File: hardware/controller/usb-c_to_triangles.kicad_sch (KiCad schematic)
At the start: 14 parts, among them J1 USB_C_Receptacle_USB2.0_16P, J2 USB_C_Receptacle_USB2.0_16P, U5 SN74LVC1T45DBV, U6 SN74LVC1T45DBV

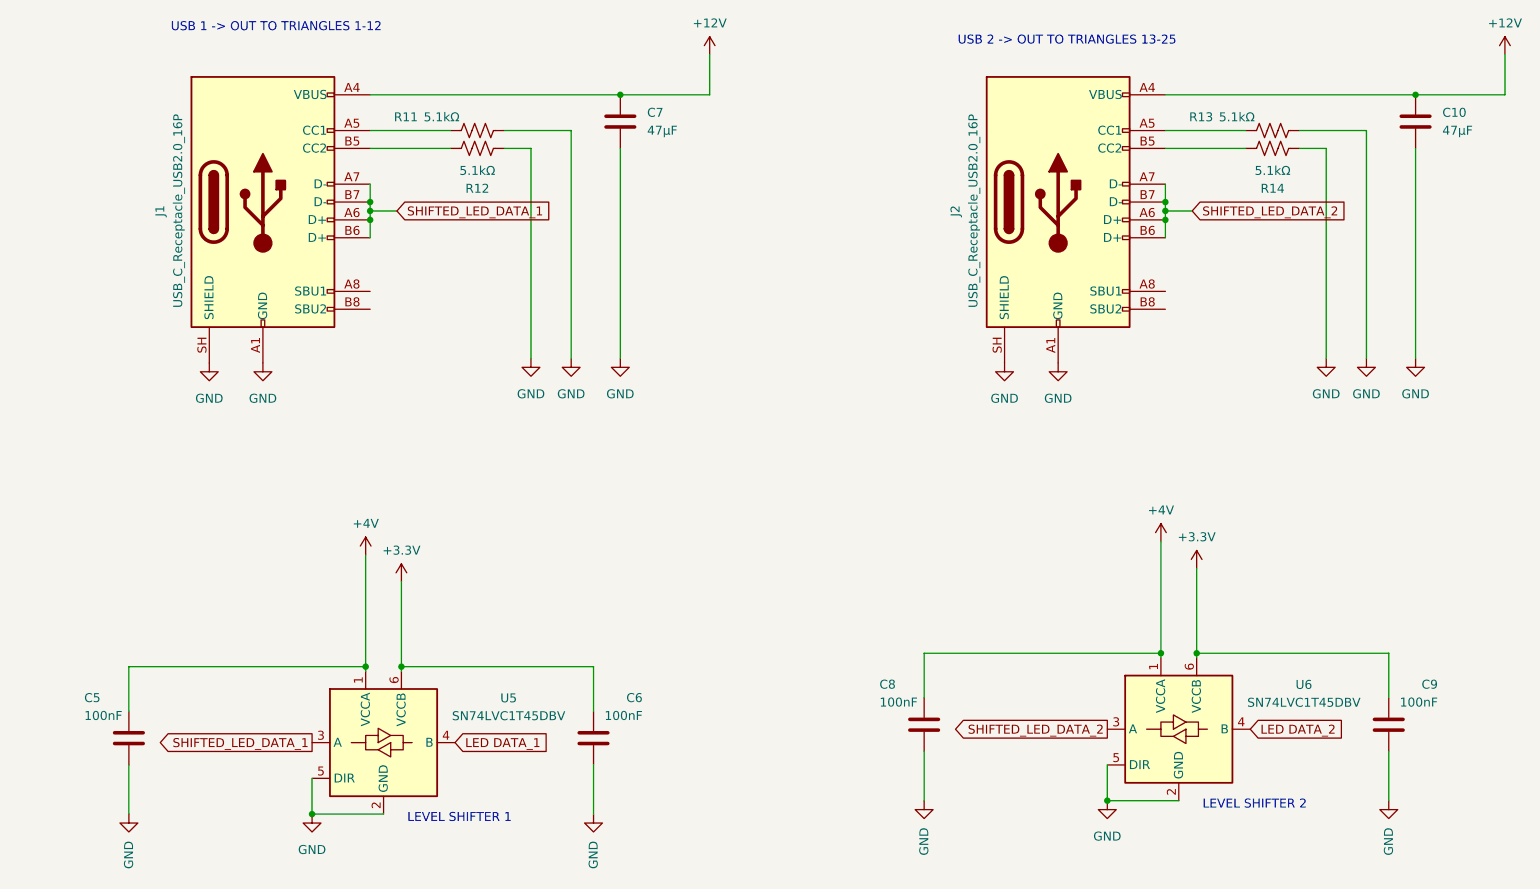
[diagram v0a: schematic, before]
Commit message: updating symbols and board
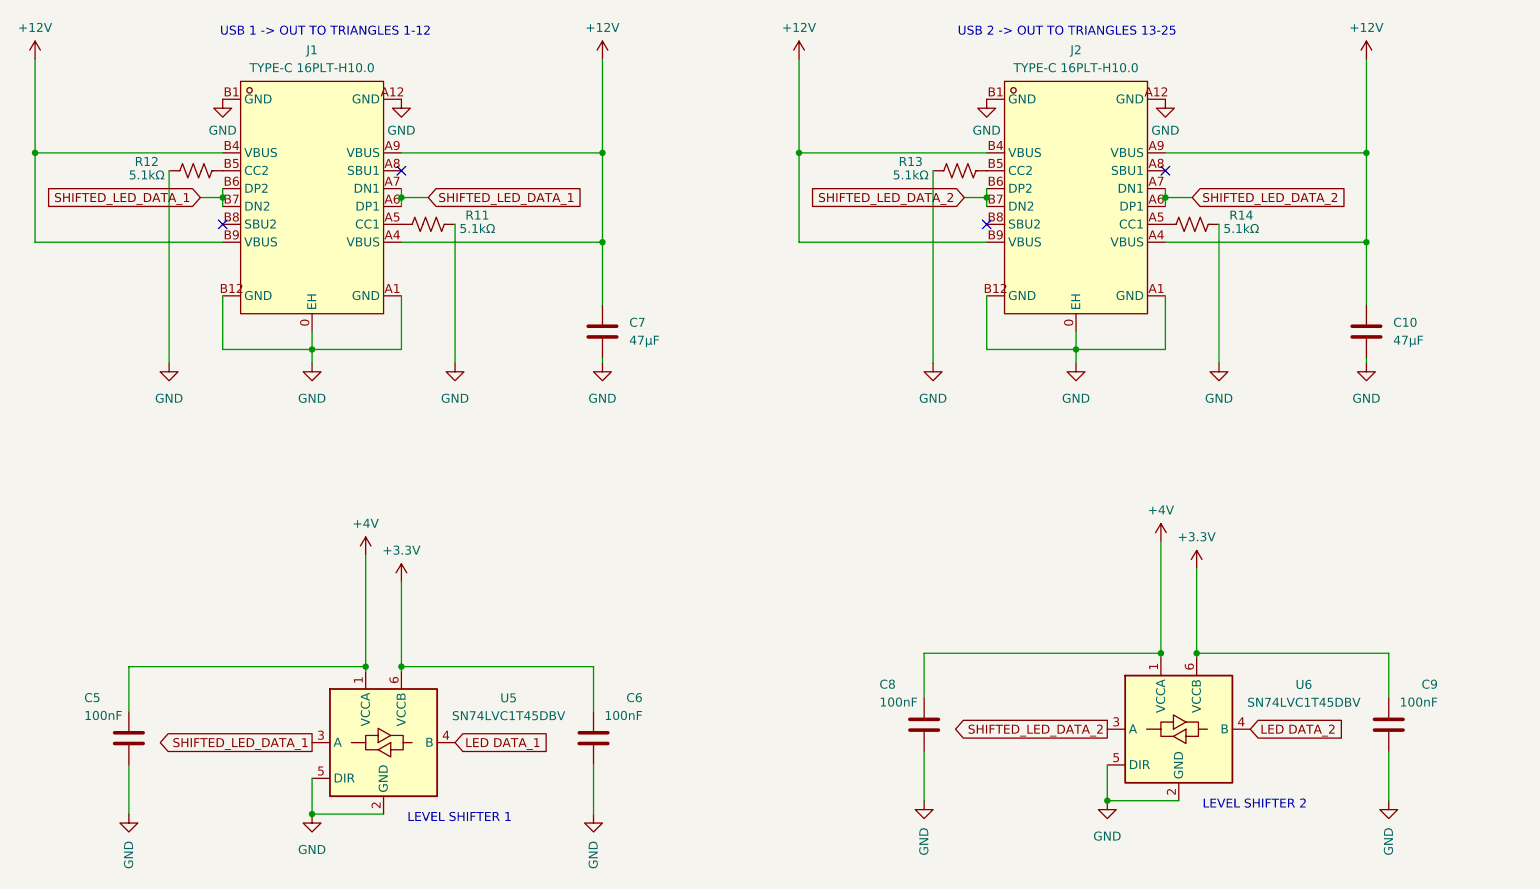
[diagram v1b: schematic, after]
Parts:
- removed J2: USB_C_Receptacle_USB2.0_16P, easyeda2kicad:TYPE-C-SMD_USB4120-03-C, symbol Connector:USB_C_Receptacle_USB2.0_16P
- added J2: TYPE-C 16PLT-H10.0, easyeda2kicad:TYPE-C-SMD_USB4120-03-C, symbol easyeda2kicad:TYPE-C16PLT-H10.0
- J1: value USB_C_Receptacle_USB2.0_16P -> TYPE-C 16PLT-H10.0; symbol Connector:USB_C_Receptacle_USB2.0_16P -> easyeda2kicad:TYPE-C16PLT-H10.0
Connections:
- net +12V: now also J2.A4 (VBUS), J2.A9 (VBUS), J2.B4 (VBUS), J2.B9 (VBUS)
- net GND: now also J1.0 (EH), R12.2, R13.2, J2.0 (EH), J2.A1 (GND), J2.A12 (GND), J2.B1 (GND), J2.B12 (GND); no longer J1.SH (SHIELD), R12.1, R13.1
- net SHIFTED_LED_DATA_2: now also J2.A6 (DP1), J2.A7 (DN1), J2.B6 (DP2), J2.B7 (DN2)
- net at R14.2: now also J2.A5 (CC1)
- net at J1.B5 (CC2): now also R12.1; no longer R12.2
- new net: J2.B5 (CC2), R13.1
- no-connect marks 0 -> 4
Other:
- moved on the sheet: C7, R11, R12
